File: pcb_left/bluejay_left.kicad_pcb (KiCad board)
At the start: 2 copper layers, 17.2 x 1.3 mm, 72 parts, among them J1 SJ-43514, U1 ATmega328P-PU, Y1 16MHz

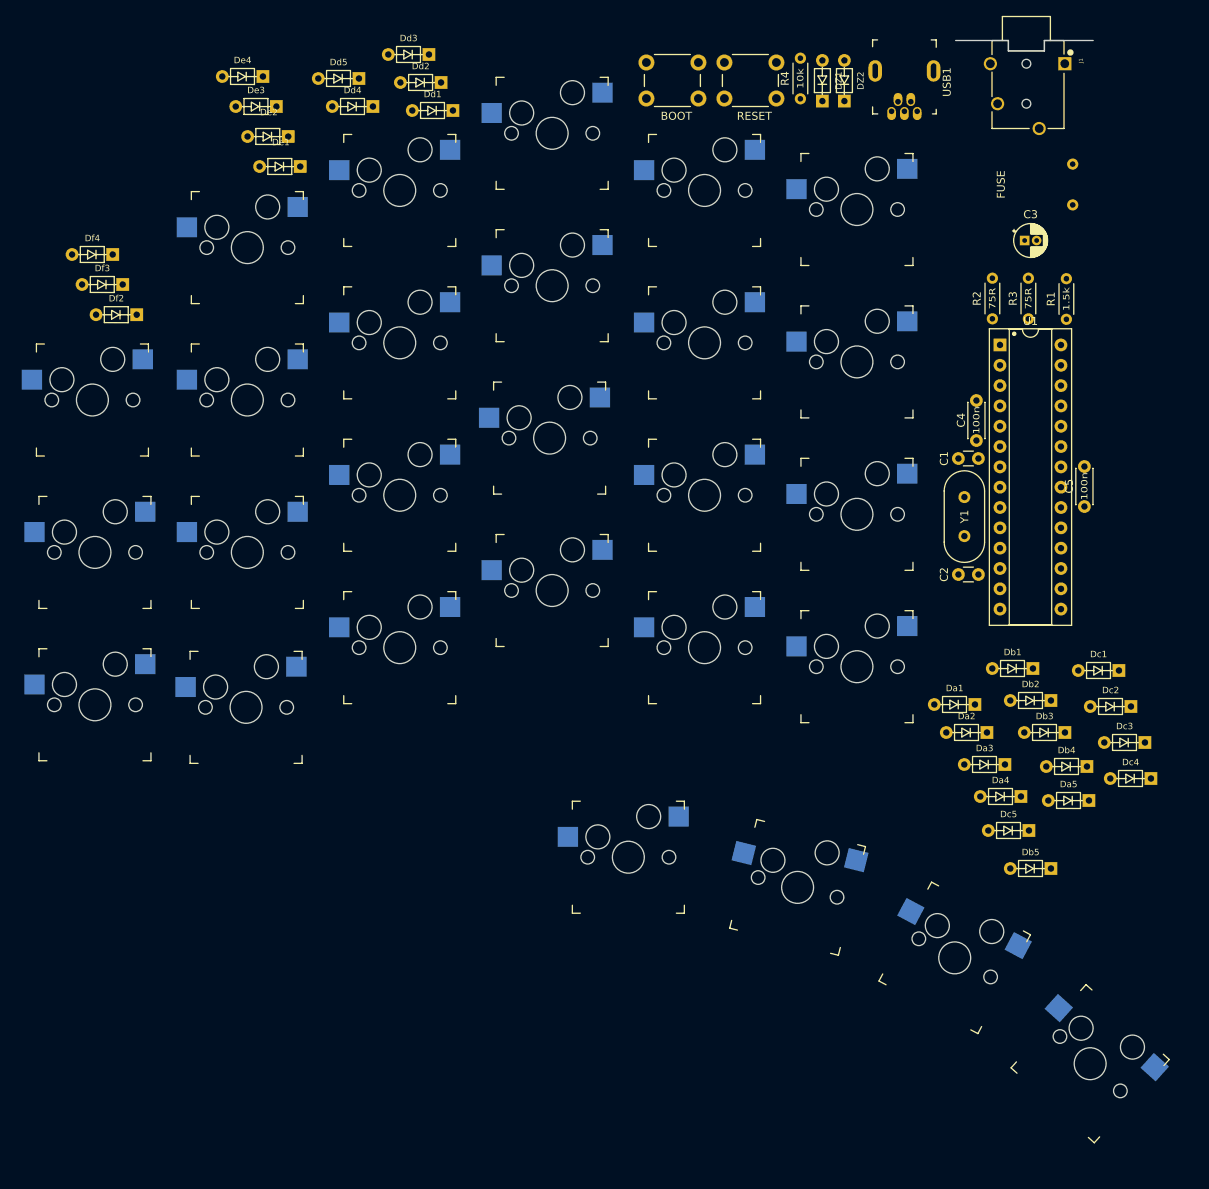
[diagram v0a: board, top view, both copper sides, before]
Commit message: Further work on pcbs
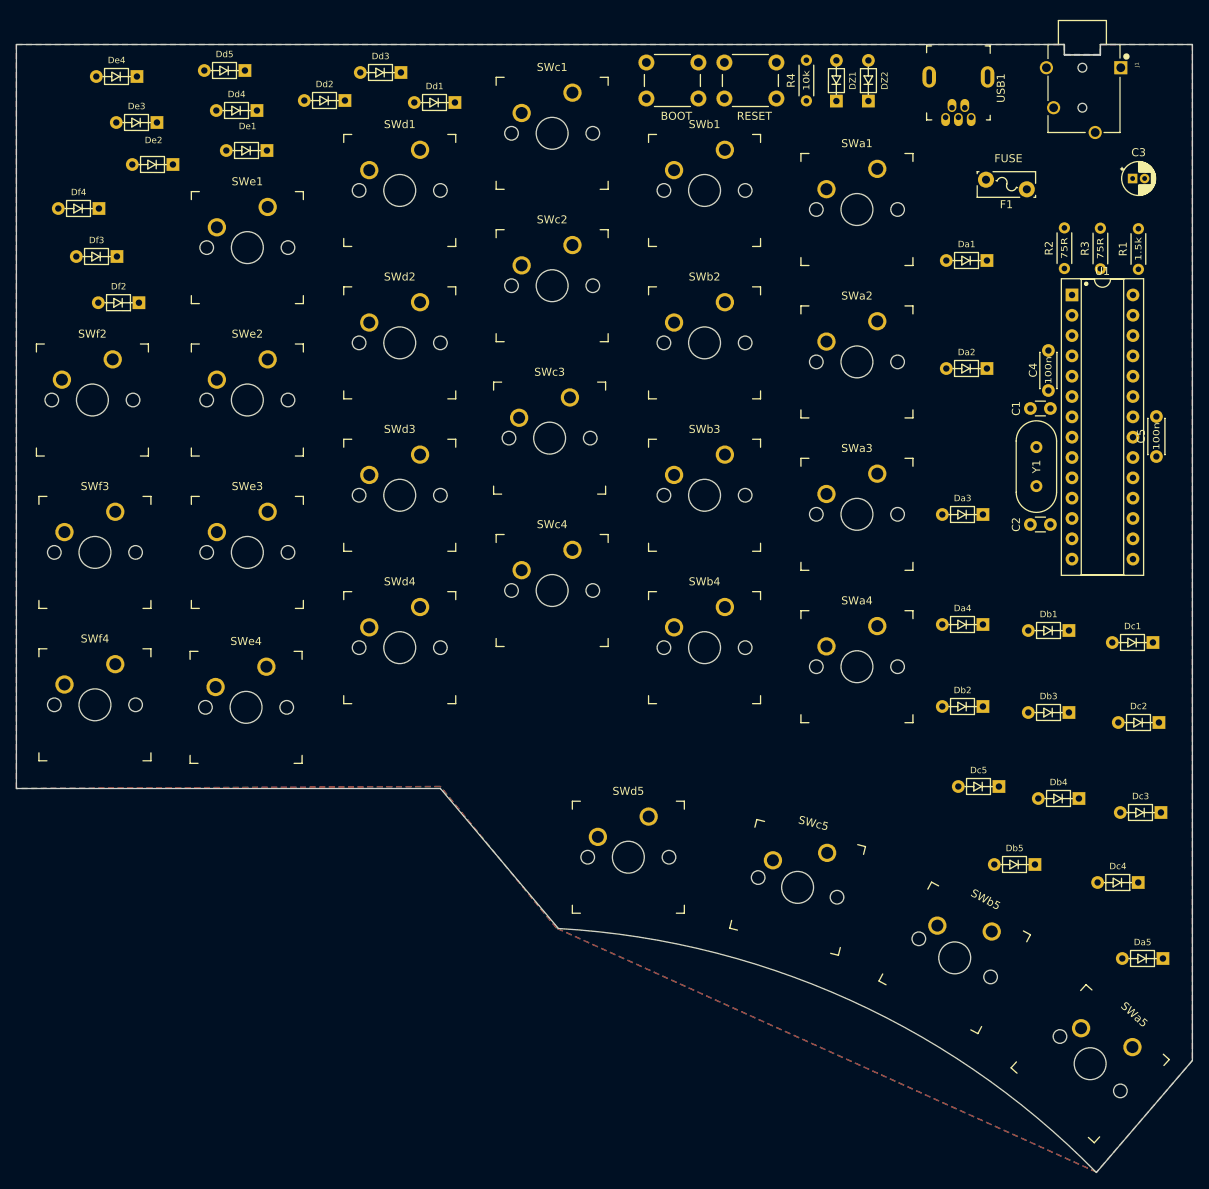
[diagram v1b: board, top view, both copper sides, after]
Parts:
- F1: footprint BlueJay footprints:polyfuse_5.1mm -> Fuse_AKL:Fuse_Bourns_MF-RG300
- SWa1, SWa2, SWa3, SWa4, SWa5, SWb1, SWb2, SWb3, SWb4, SWb5, SWc1, SWc2, SWc3, SWc4, SWc5, SWd1, SWd2, SWd3, SWd4, SWd5, SWe1, SWe2, SWe3, SWe4, SWf2, SWf3, SWf4: footprint BlueJay footprints:Kailh_socket_MX -> BlueJay footprints:SW_MX
- moved Da1 55.5 mm to (186.6, 54.0)
- moved Da2 45.5 mm to (186.6, 67.5)
- moved Da3 31.4 mm to (186.1, 85.8)
- moved Da4 22.0 mm to (186.1, 99.5)
- moved Da5 21.8 mm to (208.6, 141.2)
- moved De4 15.8 mm to (80.3, 31.0)
- moved C3 15.6 mm to (203.5, 43.8)
- moved De3 15.1 mm to (82.8, 36.8)
- moved De2 14.8 mm to (84.8, 42.0)
- moved Dd4 14.5 mm to (95.3, 35.2)
- moved Dd5 14.3 mm to (93.8, 30.2)
- moved Dc4 13.1 mm to (205.5, 131.8)
- moved Dd2 12.2 mm to (106.3, 34.0)
- moved R2 11.0 mm to (195.0, 55.0)
- moved U1 11.0 mm to (195.9, 58.3)
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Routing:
- added copper zone on B.Cu, net GND
- added copper zone on F.Cu, net GND
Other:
- board size 17.2 x 1.3 mm -> 147 x 141 mm
